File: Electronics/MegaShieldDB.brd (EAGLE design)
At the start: 100.3 x 80 mm, 45 parts, among them IC2 MCP4802, IC3 MCP4802, IC4 4013N, Q1 BF199, Q5 BF199, X1 Panel, X2 Cruise, X3 Motor, X4 Steer, X5 Brake

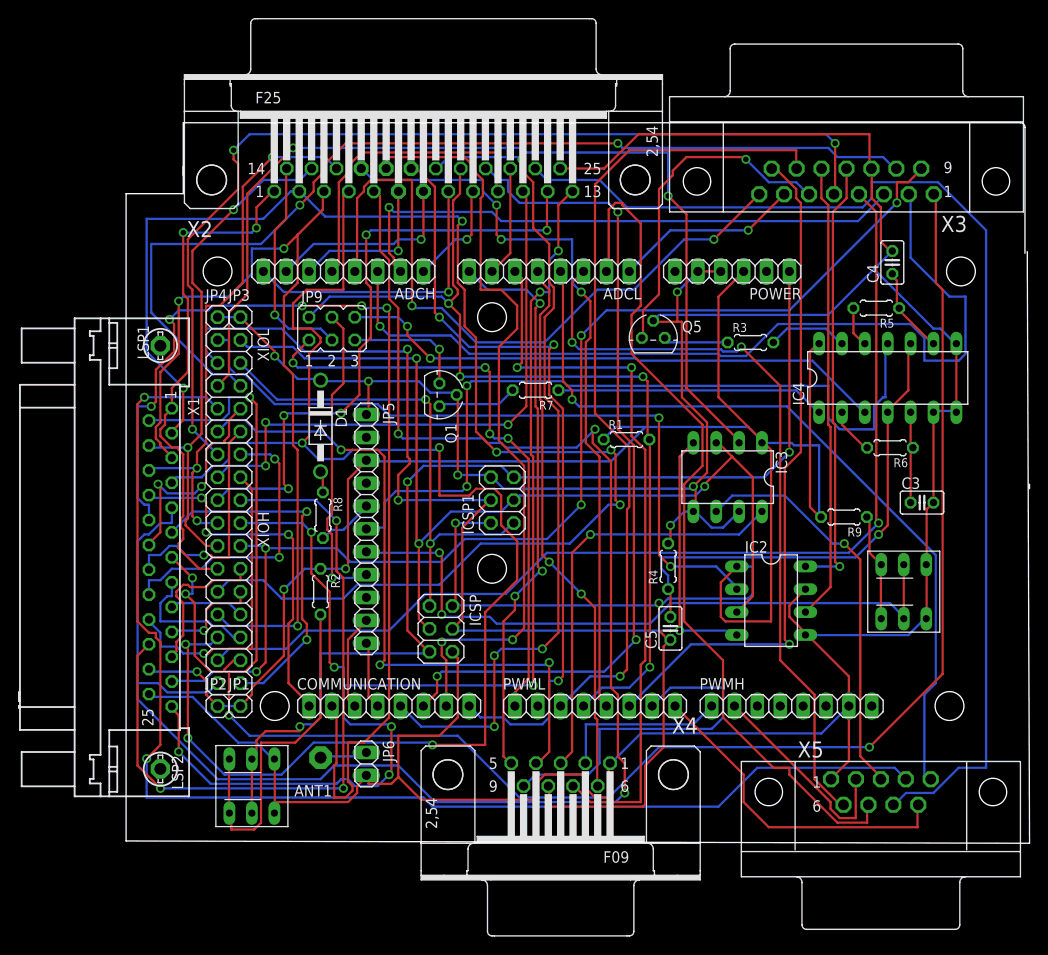
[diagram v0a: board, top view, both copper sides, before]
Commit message: noon changes of board design
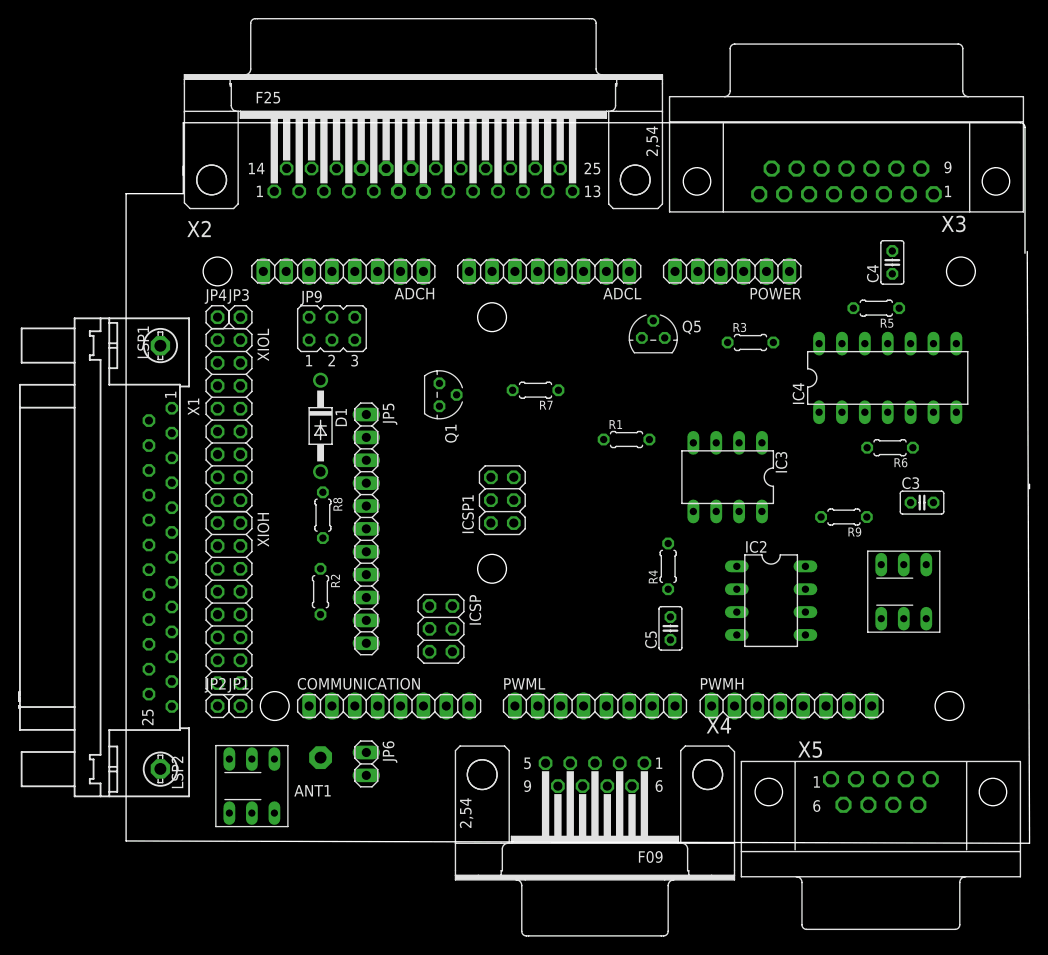
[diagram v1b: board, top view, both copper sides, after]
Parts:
- moved X4 3.81 mm to (52.1, 7.62)
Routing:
- net GND: track 405.4 -> 0.00 mm, vias 6 -> 0
- net +5V: track 279.3 -> 0.00 mm, vias 5 -> 0
- net FUEL: track 193.7 -> 0.00 mm, vias 3 -> 0
- net D23: track 187.6 -> 0.00 mm, vias 3 -> 0
- net D27: track 163.5 -> 0.00 mm, vias 5 -> 0
- net D31: track 161.1 -> 0.00 mm, vias 5 -> 0
- net D36: track 152.0 -> 0.00 mm, vias 8 -> 0
- net D47: track 142.6 -> 0.00 mm, vias 2 -> 0
- net D34: track 130.8 -> 0.00 mm, vias 5 -> 0
- net 5VBRK: track 127.9 -> 0.00 mm
- net D51: track 125.2 -> 0.00 mm, vias 3 -> 0
- net RESET: track 120.9 -> 0.00 mm, vias 3 -> 0
- net D20INT4: track 120.4 -> 0.00 mm, vias 5 -> 0
- net D25: track 117.1 -> 0.00 mm, vias 1 -> 0
- net D52: track 111.4 -> 0.00 mm, vias 3 -> 0
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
